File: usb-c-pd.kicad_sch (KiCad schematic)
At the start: 4 parts, among them J1 USB_C_Receptacle_PowerOnly_6P, J2 Barrel_Jack, U1 CYPD3177-24LQ, U2 STM32G030K8Tx

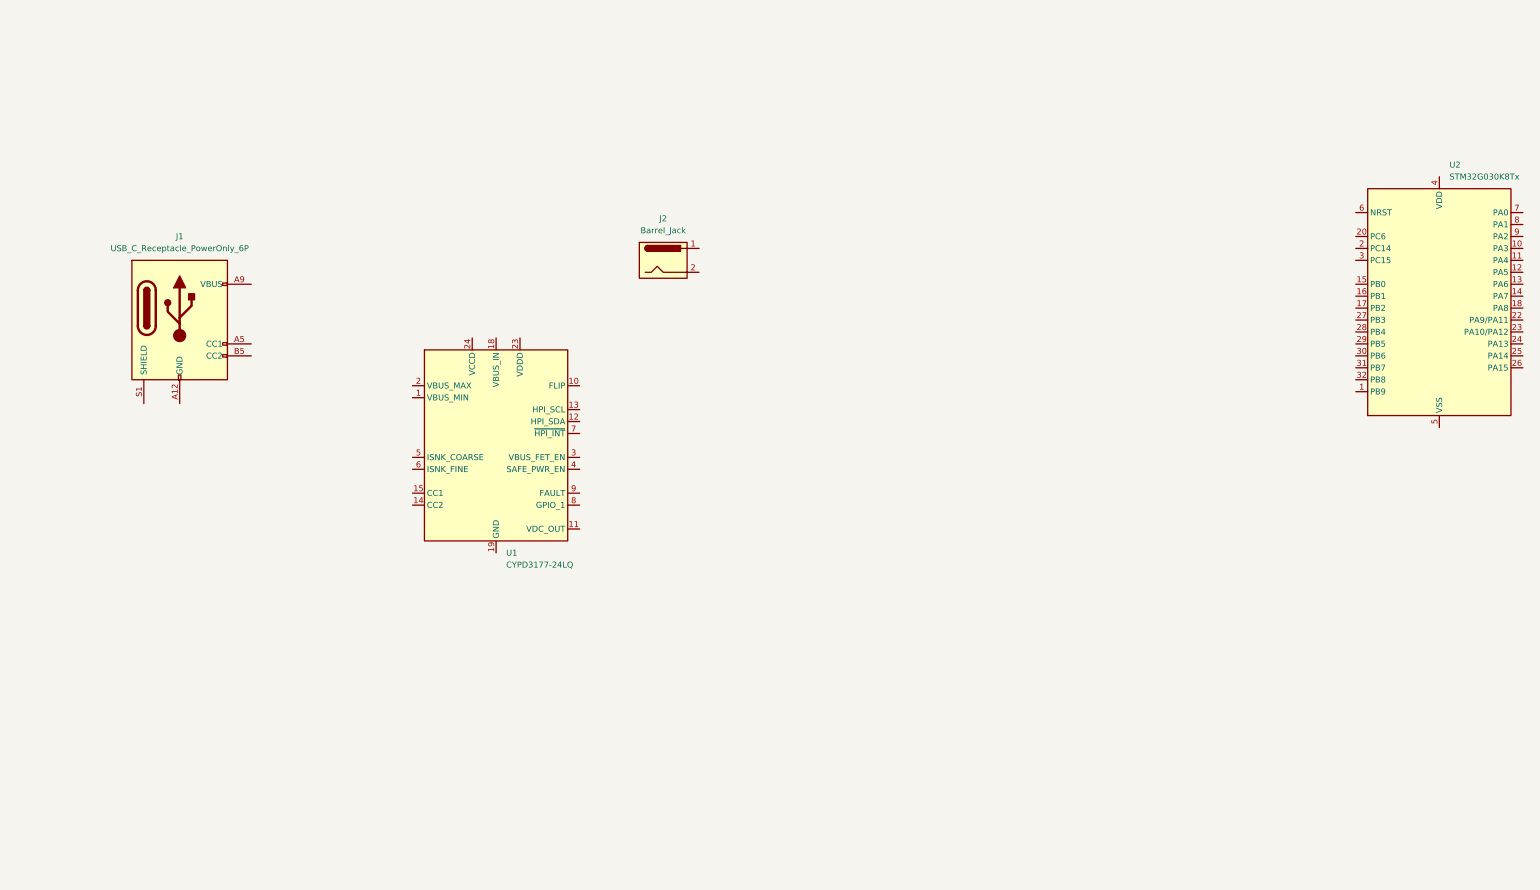
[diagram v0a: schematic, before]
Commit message: feat: ez-pd
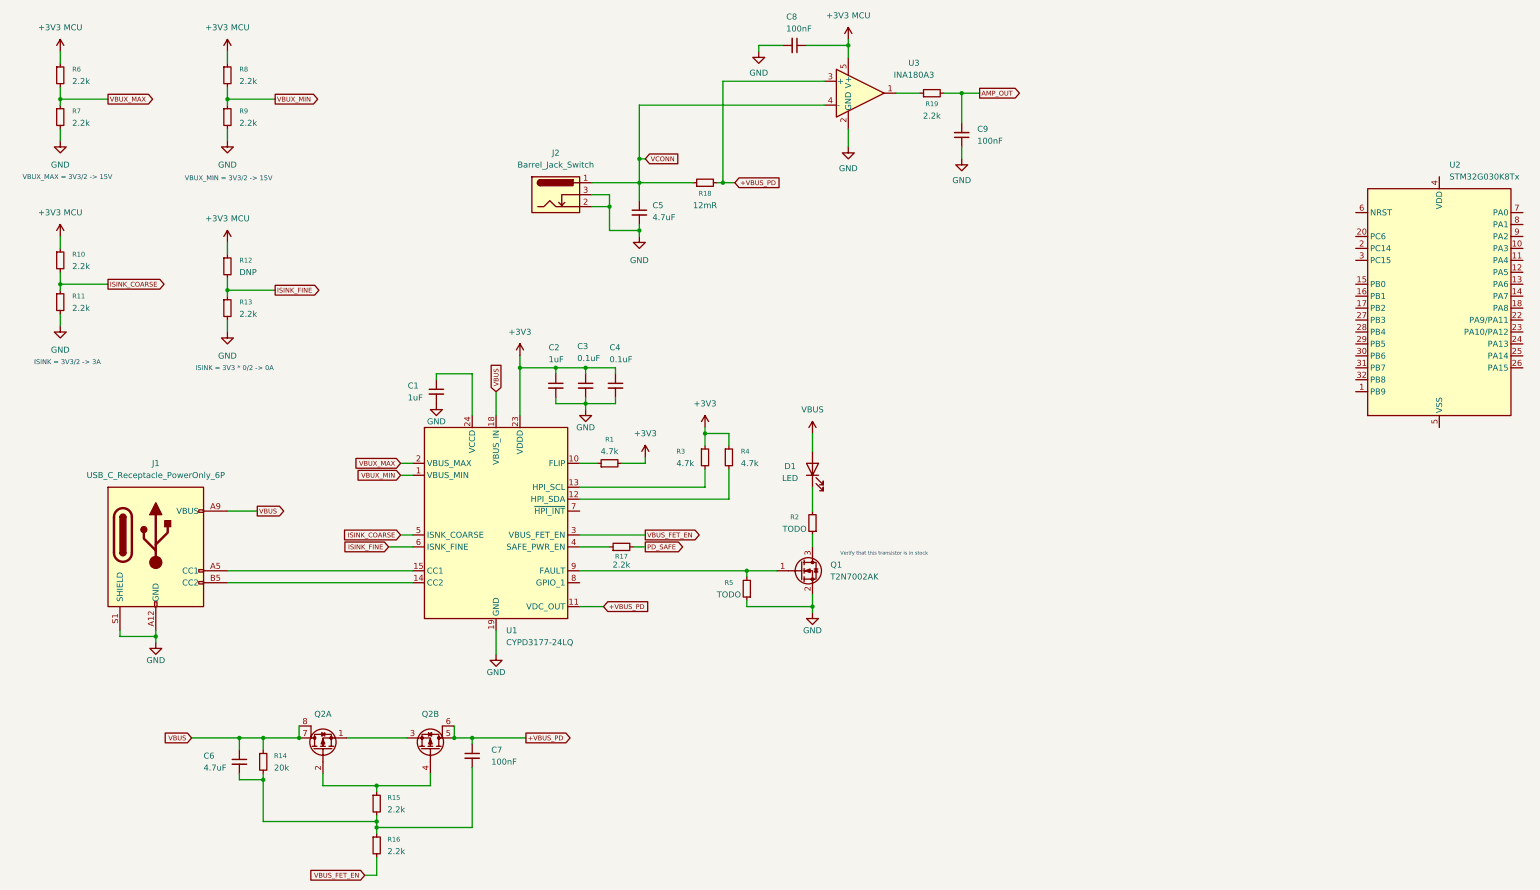
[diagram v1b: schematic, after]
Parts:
- removed J2: Barrel_Jack, symbol Connector:Barrel_Jack
- added C1, C2: 1uF, symbol Device:C_Small
- added C3, C4: 0.1uF, symbol Device:C_Small
- added C5, C6: 4.7uF, symbol Device:C_Small
- added C7, C8, C9: 100nF, symbol Device:C_Small
- added D1: LED, symbol Device:LED
- added J2: Barrel_Jack_Switch, symbol Connector:Barrel_Jack_Switch
- added Q1: T2N7002AK, Package_TO_SOT_SMD:SOT-23, symbol Transistor_FET:T2N7002AK
- added Q2: ~, usb-c-pd-lib:SOIC127P600X175-8N, symbol usb-c-pd-prodj-lib:DMP3098LSD-13
- added R1, R3, R4: 4.7k, symbol Device:R_Small
- added R10, R11, R13, R15, R16, R17, R19, R6, R7, R8, R9: 2.2k, symbol Device:R_Small
- added R12: DNP, symbol Device:R_Small
- added R14: 20k, symbol Device:R_Small
- added R18: 12mR, symbol Device:R_Small
- added R2, R5: TODO, symbol Device:R_Small
- added U3: INA180A3, Package_TO_SOT_SMD:SOT-23-5, symbol Amplifier_Current:INA180A3
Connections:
- net VBUX_MIN: now reaches U1.1 (VBUS_MIN)
- net VBUX_MIN: now also R8.2, R9.1
- net at U1.10 (FLIP): now also R1.1
- net +VBUS_PD: now reaches U1.11 (VDC_OUT)
- net +VBUS_PD: now also C7.1, Q2.5 (D2), Q2.6 (D2), R18.2, U3.3 (+)
- net at U1.12 (HPI_SDA): now also R4.2
- net at U1.13 (HPI_SCL): now also R3.2
- net at U1.14 (CC2): now also J1.B5 (CC2)
- net at U1.15 (CC1): now also J1.A5 (CC1)
- net VBUS: now reaches U1.18 (VBUS_IN)
- net VBUS: now also J1.A9 (VBUS), J1.B9 (VBUS), C6.1, D1.2 (A), Q2.7 (D), Q2.8 (D), R14.1
- net GND: now reaches U1.19 (GND), U1.22 (GND), U1.25 (GND)
- net GND: now also J1.A12 (GND), J1.B12 (GND), J1.S1 (SHIELD), C1.2, C2.2, C3.2, C4.2, C5.2, C8.2, C9.1, J2.2, J2.3, Q1.2 (S), R11.2, R13.2, R5.1, R7.2, R9.2, U3.2 (GND)
- net VBUX_MAX: now reaches U1.2 (VBUS_MAX)
- net VBUX_MAX: now also R6.2, R7.1
- net +3V3: now reaches U1.23 (VDDD)
- net +3V3: now also C2.1, C3.1, C4.1, R1.2, R3.1, R4.1
- net at U1.24 (VCCD): now also C1.1
- net VBUS_FET_EN: now reaches U1.3 (VBUS_FET_EN)
- net VBUS_FET_EN: now also R16.2
- net at U1.4 (SAFE_PWR_EN): now also R17.1
- net ISINK_COARSE: now reaches U1.5 (ISNK_COARSE)
- net ISINK_COARSE: now also R10.2, R11.1
- net ISINK_FINE: now reaches U1.6 (ISNK_FINE)
- net ISINK_FINE: now also R12.2, R13.1
- net at U1.9 (FAULT): now also Q1.1 (G), R5.2
- new net: Q1.3 (D), R2.1
- new net: Q2.1 (S1), Q2.3 (S2)
- new net: Q2.2 (G1), Q2.4 (G2), R15.1
- new net: D1.1 (K), R2.2
- new net: R19.1, U3.1
- new net: C6.2, C7.2, R14.2, R15.2, R16.1
- new net +3V3 MCU: C8.1, R10.1, R12.1, R6.1, R8.1, U3.5 (V+)
- new net AMP_OUT: C9.2, R19.2
- new net PD_SAFE: R17.2
- new net VCONN: C5.1, J2.1, R18.1, U3.4 (-)
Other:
- note added: "ISINK = 3V3 * 0/2 -> 0A"
- note added: "ISINK = 3V3/2 -> 3A"
- note added: "VBUX_MAX = 3V3/2 -> 15V"
- note added: "VBUX_MIN = 3V3/2 -> 15V"
- note added: "Verify that this transistor is in stock"
- moved on the sheet: J1, U1
